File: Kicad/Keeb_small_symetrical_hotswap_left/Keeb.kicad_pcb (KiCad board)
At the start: 2 copper layers, 96.6 x 97.5 mm, 30 parts, among them J1 TYPE-C-31-M-12, SW1 CherryMX, SW10 CherryMX, SW11 CherryMX, SW13 CherryMX, SW14 CherryMX, SW15 CherryMX, SW16 CherryMX, SW17 CherryMX, SW18 CherryMX, SW19 CherryMX, SW2 CherryMX, SW20 CherryMX, SW3 CherryMX, SW4 CherryMX, SW5 CherryMX, SW6 CherryMX, SW7 CherryMX, SW8 CherryMX, SW9 CherryMX, U1 Pico, U2 KY-040

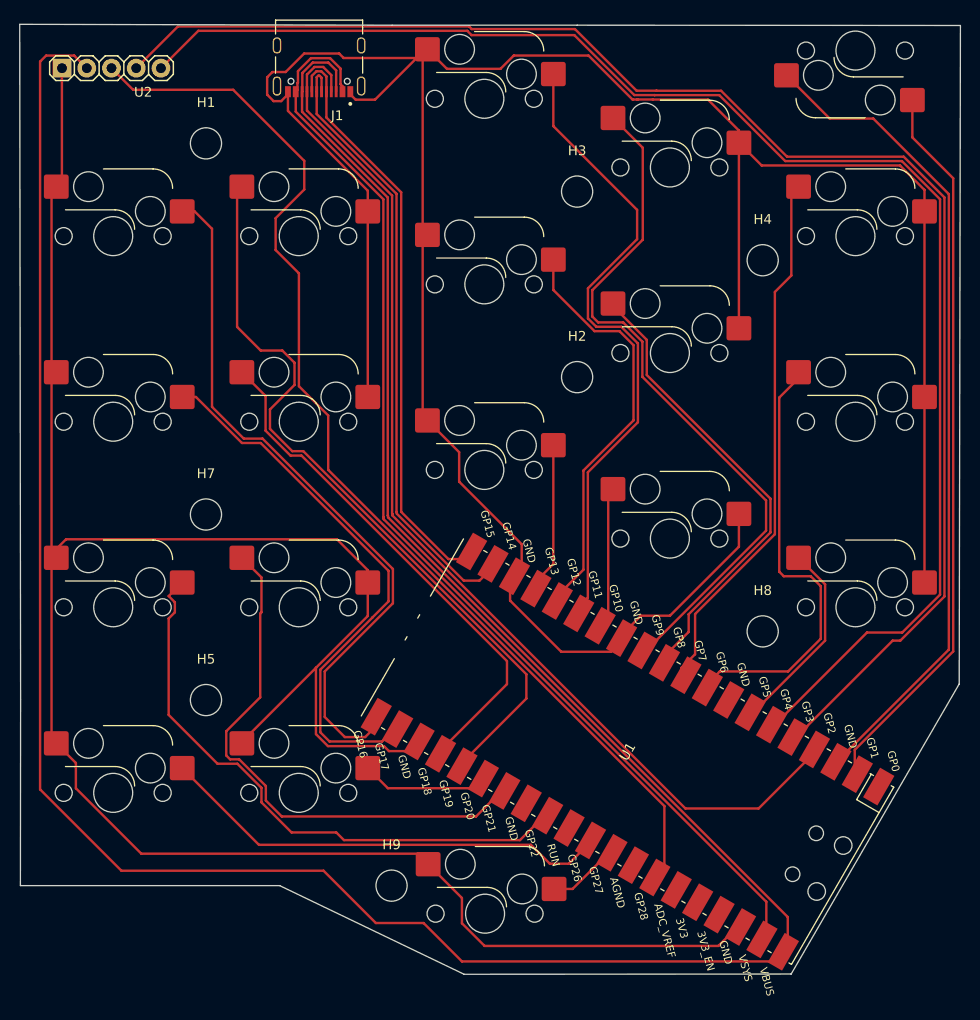
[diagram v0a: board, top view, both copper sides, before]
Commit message: Worked a bit on the edge-cuts
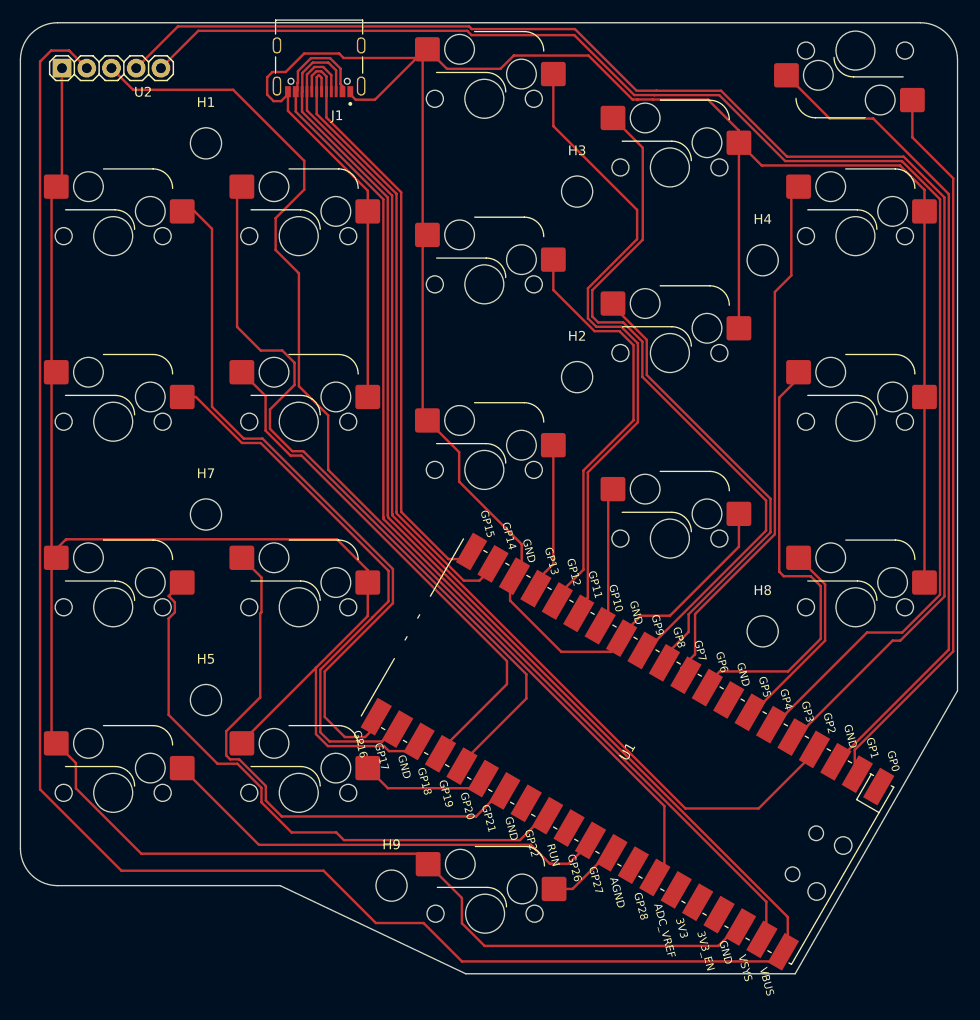
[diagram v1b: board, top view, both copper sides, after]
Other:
- board size 96.6 x 97.5 mm -> 96.2 x 97.6 mm
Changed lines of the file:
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@@
     )
   )
-  (gr_poly
-    (pts
-      (xy 199.1 33.992944)
-      (xy 159.76 33.962944)
-      (xy 140.76 33.962944)
-      (xy 102.53 33.872944)
-      (xy 102.62 103.232944)
-      (xy 102.6 122.292944)
-      (xy 129.22 122.292944)
-      (xy 148.15 131.392944)
-      (xy 181.725 131.367944)
-      (xy 198.975 101.592944)
-    )
-    (stroke (width 0.05) (type solid)) (fill none) (layer "Edge.Cuts"))
+  (gr_line (start 102.6 37.520444) (end 102.6 118.482944)
+    (stroke (width 0.05) (type default)) (layer "Edge.Cuts"))
+  (gr_line (start 198.8025 102.290444) (end 198.8025 37.520444)
+    (stroke (width 0.05) (type default)) (layer "Edge.Cuts"))
+  (gr_line (start 148.32 131.341694) (end 182.13375 131.341694)
+    (stroke (width 0.05) (type default)) (layer "Edge.Cuts"))
+  (gr_arc (start 102.6 37.520444) (mid 103.715923 34.826367) (end 106.41 33.710444)
+    (stroke (width 0.05) (type default)) (layer "Edge.Cuts"))
+  (gr_line (start 194.9925 33.710444) (end 106.41 33.710444)
+    (stroke (width 0.05) (type default)) (layer "Edge.Cuts"))
+  (gr_line (start 129.27 122.292944) (end 148.32 131.341694)
+    (stroke (width 0.05) (type default)) (layer "Edge.Cuts"))
+  (gr_arc (start 194.9925 33.710444) (mid 197.686577 34.826367) (end 198.8025 37.520444)
+    (stroke (width 0.05) (type default)) (layer "Edge.Cuts"))
+  (gr_line (start 106.41 122.292944) (end 129.27 122.292944)
+    (stroke (width 0.05) (type default)) (layer "Edge.Cuts"))
+  (gr_arc (start 106.41 122.292944) (mid 103.715923 121.177021) (end 102.6 118.482944)
+    (stroke (width 0.05) (type default)) (layer "Edge.Cuts"))
+  (gr_line (start 182.13375 131.341694) (end 198.8025 102.290444)
+    (stroke (width 0.05) (type default)) (layer "Edge.Cuts"))
   (segment (start 179.15 82.75934) (end 179.15 85.848312) (width 0.25) (layer "F.Cu") (net 1))
   (segment (start 166.49 46.544944) (end 166.49 55.982944) (width 0.25) (layer "F.Cu") (net 1))
@@
   (segment (start 138.26 50.952944) (end 130.065 42.757944) (width 0.25) (layer "F.Cu") (net 15))
   (segment (start 135.095 86.737944) (end 107.285 86.737944) (width 0.25) (layer "F.Cu") (net 15))
-  (segment (start 104.62 112.412944) (end 112.97 120.762944) (width 0.25) (layer "F.Cu") (net 16))
   (segment (start 140.31 51.646448) (end 131.515 42.851448) (width 0.25) (layer "F.Cu") (net 16))
   (segment (start 140.34 84.482219) (end 140.34 84.32736) (width 0.25) (layer "F.Cu") (net 16))
-  (segment (start 133.72 120.762944) (end 139.09 126.132944) (width 0.25) (layer "F.Cu") (net 16))
+  (segment (start 105.755 36.567944) (end 104.62 37.702944) (width 0.25) (layer "F.Cu") (net 16))
   (segment (start 131.515 42.851448) (end 131.515 40.79) (width 0.25) (layer "F.Cu") (net 16))
   (segment (start 140.34 84.32736) (end 140.31 84.29736) (width 0.25) (layer "F.Cu") (net 16))
   (segment (start 135.015 38.605812) (end 135.015 40.79) (width 0.25) (layer "F.Cu") (net 16))
+  (segment (start 133.72 120.762944) (end 139.09 126.132944) (width 0.25) (layer "F.Cu") (net 16))
+  (segment (start 109.41 38.372944) (end 107.605 36.567944) (width 0.25) (layer "F.Cu") (net 16))
   (segment (start 131.54 38.870812) (end 132.610812 37.8) (width 0.25) (layer "F.Cu") (net 16))
-  (segment (start 104.62 37.702944) (end 104.62 112.412944) (width 0.25) (layer "F.Cu") (net 16))
-  (segment (start 143.99 126.132944) (end 147.930877 130.073821) (width 0.25) (layer "F.Cu") (net 16))
+  (segment (start 104.62 112.412944) (end 112.97 120.762944) (width 0.25) (layer "F.Cu") (net 16))
   (segment (start 131.515 40.79) (end 131.54 40.765) (width 0.25) (layer "F.Cu") (net 16))
-  (segment (start 140.31 84.29736) (end 140.31 51.646448) (width 0.25) (layer "F.Cu") (net 16))
   (segment (start 112.97 120.762944) (end 133.72 120.762944) (width 0.25) (layer "F.Cu") (net 16))
   (segment (start 139.09 126.132944) (end 143.99 126.132944) (width 0.25) (layer "F.Cu") (net 16))
+  (segment (start 140.31 84.29736) (end 140.31 51.646448) (width 0.25) (layer "F.Cu") (net 16))
+  (segment (start 143.99 126.132944) (end 147.930877 130.073821) (width 0.25) (layer "F.Cu") (net 16))
   (segment (start 181.37414 125.516359) (end 140.34 84.482219) (width 0.25) (layer "F.Cu") (net 16))
-  (segment (start 179.599173 130.073821) (end 181.37414 128.298854) (width 0.25) (layer "F.Cu") (net 16))
   (segment (start 181.37414 128.298854) (end 181.37414 125.516359) (width 0.25) (layer "F.Cu") (net 16))
-  (segment (start 109.41 38.372944) (end 108.1198 37.082744) (width 0.25) (layer "F.Cu") (net 16))
-  (segment (start 105.2402 37.082744) (end 104.62 37.702944) (width 0.25) (layer "F.Cu") (net 16))
+  (segment (start 104.62 37.702944) (end 104.62 112.412944) (width 0.25) (layer "F.Cu") (net 16))
   (segment (start 132.610812 37.8) (end 134.209188 37.8) (width 0.25) (layer "F.Cu") (net 16))
   (segment (start 134.209188 37.8) (end 135.015 38.605812) (width 0.25) (layer "F.Cu") (net 16))
+  (segment (start 107.605 36.567944) (end 105.755 36.567944) (width 0.25) (layer "F.Cu") (net 16))
+  (segment (start 131.54 40.765) (end 131.54 38.870812) (width 0.25) (layer "F.Cu") (net 16))
   (segment (start 147.930877 130.073821) (end 179.599173 130.073821) (width 0.25) (layer "F.Cu") (net 16))
-  (segment (start 131.54 40.765) (end 131.54 38.870812) (width 0.25) (layer "F.Cu") (net 16))
-  (segment (start 108.1198 37.082744) (end 105.2402 37.082744) (width 0.25) (layer "F.Cu") (net 16))
+  (segment (start 179.599173 130.073821) (end 181.37414 128.298854) (width 0.25) (layer "F.Cu") (net 16))
   (segment (start 188.064435 111.630922) (end 188.250853 111.444504) (width 0.25) (layer "F.Cu") (net 23))
   (segment (start 188.250853 108.356335) (end 198.36 98.247188) (width 0.25) (layer "F.Cu") (net 23))
